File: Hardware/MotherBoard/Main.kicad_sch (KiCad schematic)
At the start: 19 parts, among them J11 RDY_PULLUP, J12 NMI_PULLUP, J9 Conn_02x02_Odd_Even, SW1 RESET_SW, U2 28C256, U3 WD65C22, U4 HM62256BLP, U5 WD65C02, X1 ACO-1MHz

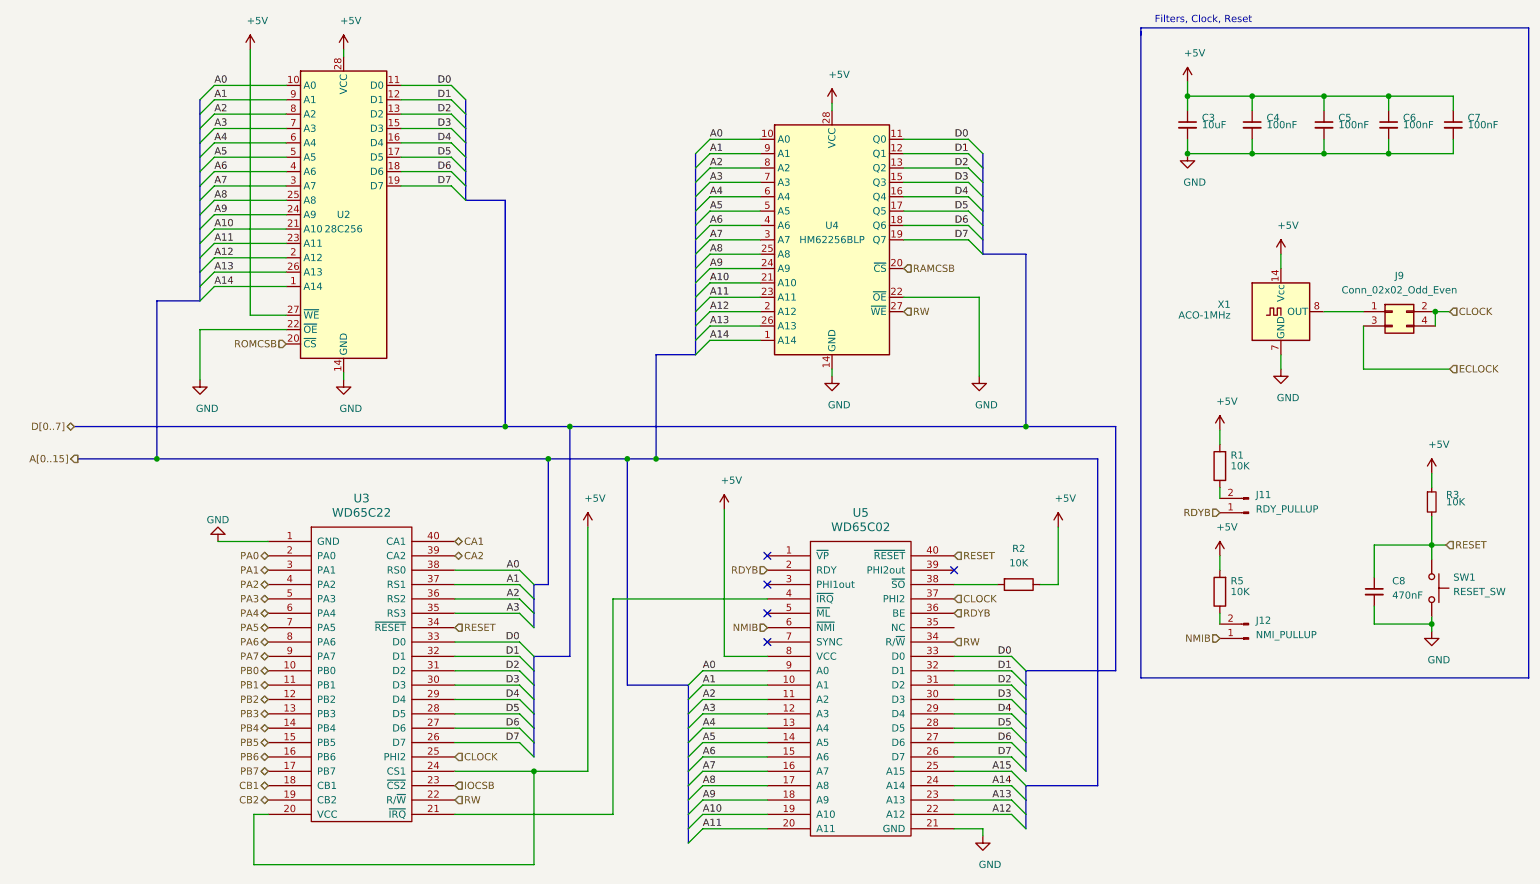
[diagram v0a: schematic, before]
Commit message: Version 1.2
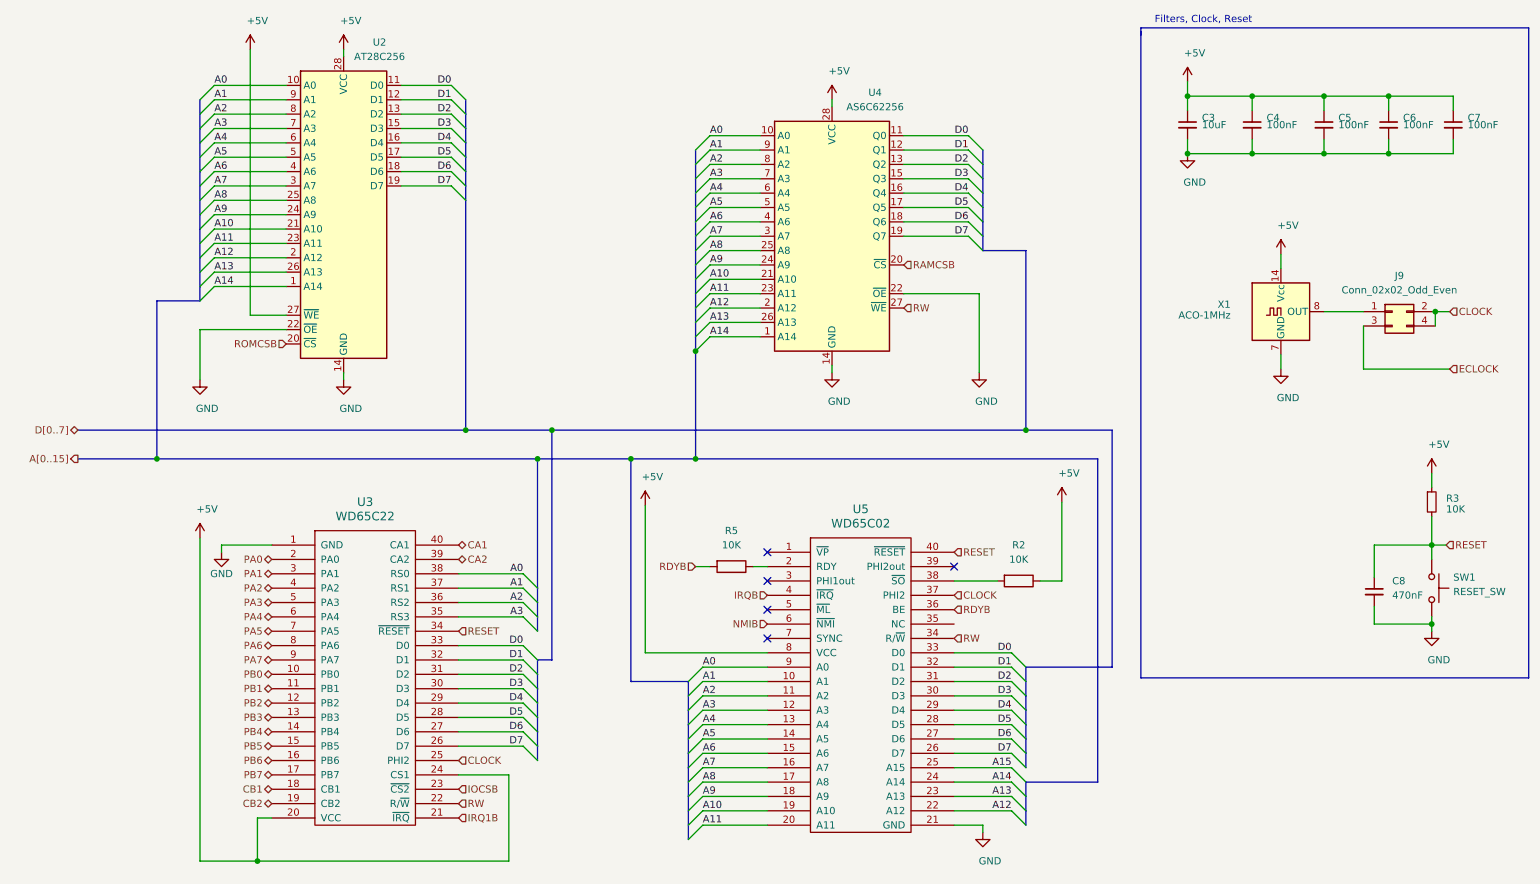
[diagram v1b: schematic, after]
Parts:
- removed J11: RDY_PULLUP, symbol Connector:Conn_01x02_Male
- removed J12: NMI_PULLUP, symbol Connector:Conn_01x02_Male
- removed R1: 10K, Resistor_THT:R_Axial_DIN0207_L6.3mm_D2.5mm_P10.16mm_Horizontal, symbol Device:R
- C8: footprint Capacitor_THT:C_Disc_D5.0mm_W2.5mm_P2.50mm -> Capacitor_THT:C_Disc_D5.0mm_W2.5mm_P5.00mm
- U2: value 28C256 -> AT28C256
- U4: value HM62256BLP -> AS6C62256
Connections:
- net +5V: no longer R5.2
- net RDYB: now also R5.2; no longer U5.2 (RDY)
- net at R5.1: now also U5.2 (RDY)
- net IRQ1B: now reaches U3.21 (~IRQ)
- net IRQ1B: no longer U5.4 (~IRQ)
- new net IRQB: U5.4 (~IRQ)
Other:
- moved on the sheet: R2, U3, U4, U5
